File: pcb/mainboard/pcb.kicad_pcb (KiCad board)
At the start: 4 copper layers, 58 x 47 mm, 193 parts, among them J201 Conn_02x05_Odd_Even, J401 FH12-40S-0.5SH, J601 USB_C_Receptacle, SW701 EVQPUJ02K, U200 XC6SLX16-FTG256, U204 SY8008, U205 SY8008, U206 SY8008, U401 TPS65185, U502 MT41K64M16TW, U601 PTN3460, U602 TPS2001D, U603 USBLC6-2P6, U604 FUSB302BMPX, U605 CBTL02043A, U701 W25Q32JV, U702 RP2040, Y201 33MHz, Y701 12MHz

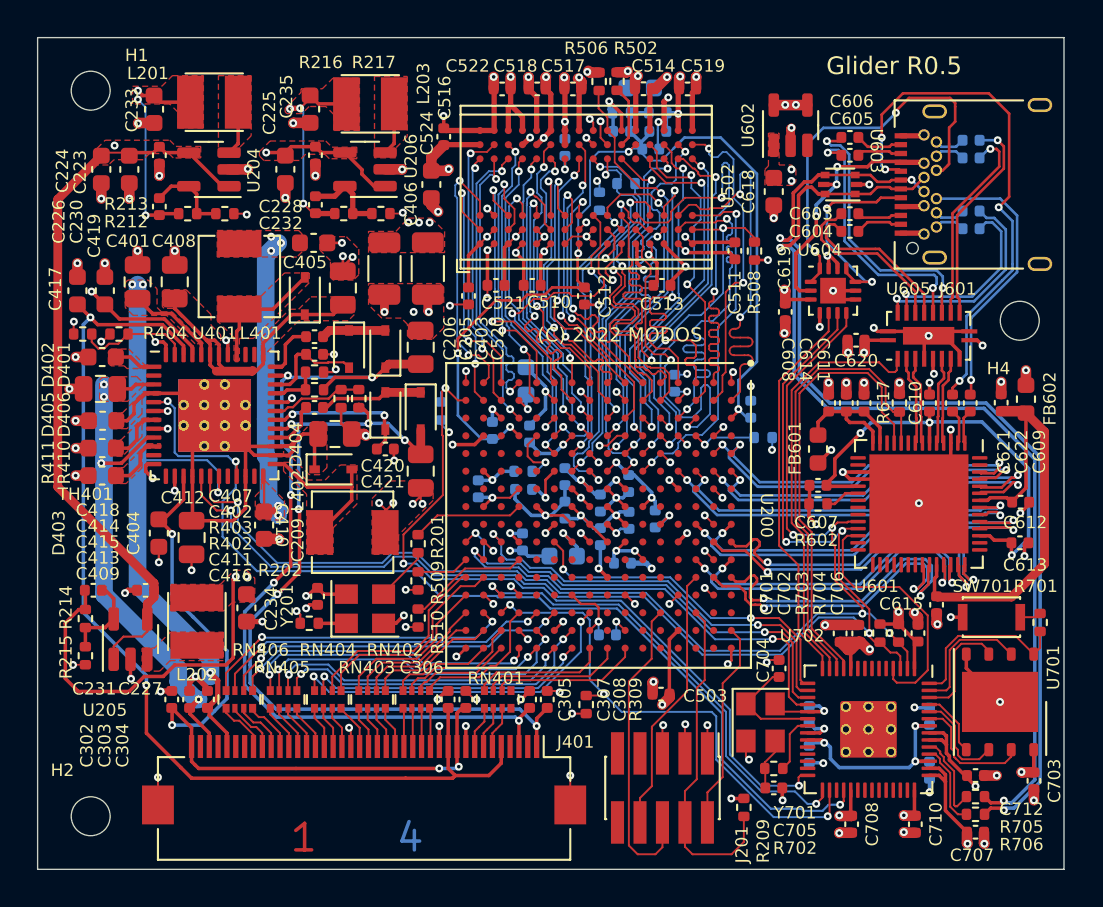
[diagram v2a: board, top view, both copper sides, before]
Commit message: pcb: r0p6
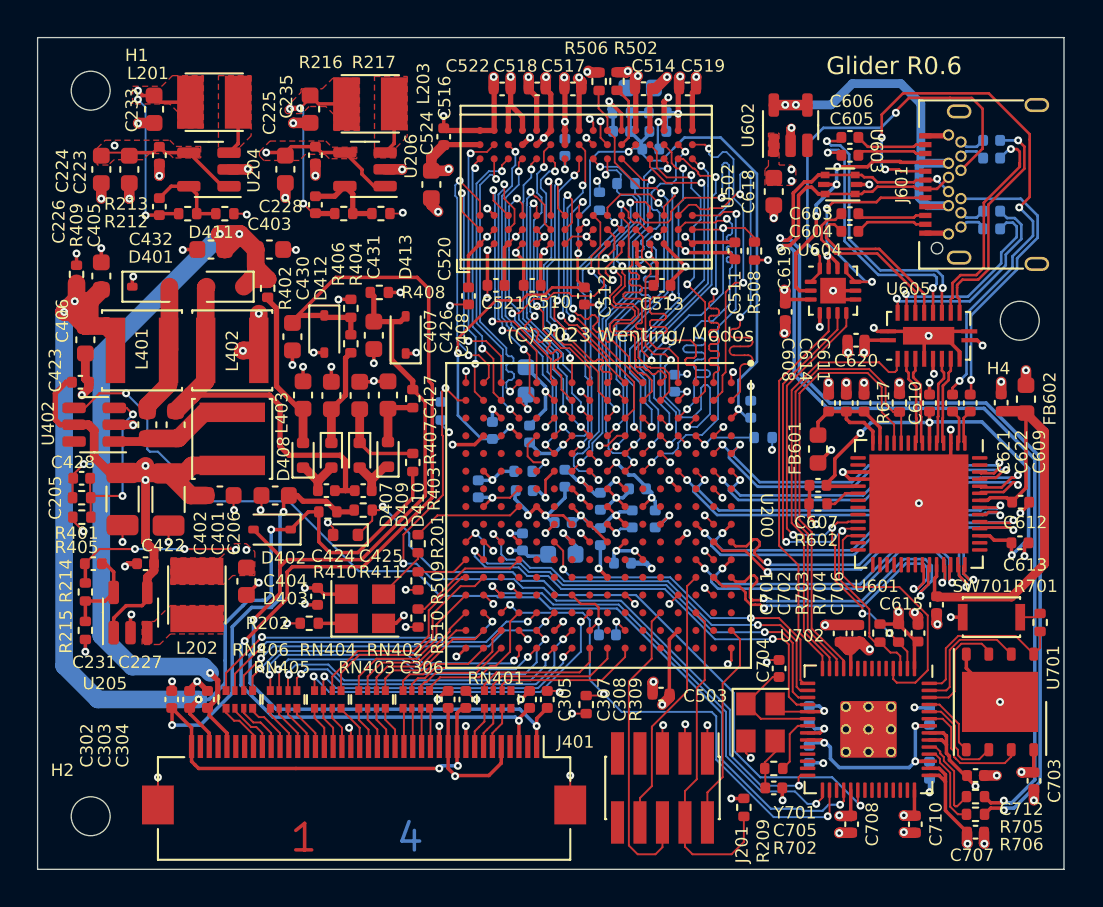
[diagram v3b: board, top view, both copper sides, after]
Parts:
- removed C409, C413, C414, C415, C417, C419: 4.7uF, Capacitor_SMD:C_0603_1608Metric
- removed C410: 10uF, Capacitor_SMD:C_0603_1608Metric
- removed C411: 10nF, Capacitor_SMD:C_0402_1005Metric
- removed C412, C416, C418, C421: 4.7uF/25V, Capacitor_SMD:C_0805_2012Metric
- removed C420: 100nF, Capacitor_SMD:C_0402_1005Metric
- removed D404, D405, D406: B0530WS, Diode_SMD:D_SOD-323
- removed TH401: 10K, Resistor_SMD:R_0402_1005Metric
- removed U401: TPS65185, footprints:QFN-48-1EP_7x7mm_P0.5mm_EP4.1x4.1mm_ThermalVias
- added C422: 10uF, Capacitor_SMD:C_0603_1608Metric, F.Cu at (110.3, 78.9)
- added C423: 100nF, Capacitor_SMD:C_0402_1005Metric, F.Cu at (102.4, 72.5)
- added C424: 10nF, Capacitor_SMD:C_0402_1005Metric, F.Cu at (116.3, 78.6)
- added C425: 10nF, Capacitor_SMD:C_0402_1005Metric, F.Cu at (118.4, 78.6)
- added C426: 1uF/50V, Capacitor_SMD:C_0603_1608Metric, F.Cu at (116.6, 73.2)
- added C427: 1uF/50V, Capacitor_SMD:C_0603_1608Metric, F.Cu at (119.8, 73.2)
- added C428: 22pF, Capacitor_SMD:C_0402_1005Metric, F.Cu at (102.5, 77.9)
- added C430: 1uF/50V, Capacitor_SMD:C_0603_1608Metric, F.Cu at (114.4, 69.9)
- added C431: 1uF/50V, Capacitor_SMD:C_0603_1608Metric, F.Cu at (119.0, 69.8)
- added C432: 10uF/25V, Capacitor_SMD:C_0603_1608Metric, F.Cu at (109.8, 65.0)
- added D407: 4148WT, Diode_SMD:D_SOD-523, F.Cu at (116.6, 76.6)
- added D408: 4148WT, Diode_SMD:D_SOD-523, F.Cu at (115.0, 76.6)
- added D409: 4148WT, Diode_SMD:D_SOD-523, F.Cu at (118.2, 76.6)
- added D410: 4148WT, Diode_SMD:D_SOD-523, F.Cu at (119.8, 76.5)
- added D411: B0530WS, Diode_SMD:D_SOD-323, F.Cu at (110.6, 67.1)
- added D412: EDZVT2R22B, Diode_SMD:D_SOD-323, F.Cu at (116.2, 69.8)
- added D413: EDZVT2R20B, Diode_SMD:D_SOD-323, F.Cu at (120.8, 69.8)
- added L403: WPN4020H2R2MT, Inductor_SMD:L_Changjiang_FNR4020S, F.Cu at (111.0, 75.7)
- added R401: 120K/1%, Resistor_SMD:R_0402_1005Metric, F.Cu at (102.5, 79.0)
- added R405: 5.1K/1%, Resistor_SMD:R_0402_1005Metric, F.Cu at (102.5, 80.1)
- added R406: 2K, Resistor_SMD:R_0402_1005Metric, F.Cu at (117.7, 70.3)
- added R407: 2K, Resistor_SMD:R_0402_1005Metric, F.Cu at (121.2, 73.4)
- added R408: 120K/1%, Resistor_SMD:R_0402_1005Metric, F.Cu at (119.3, 67.4)
- added R409: 120K/1%, Resistor_SMD:R_0402_1005Metric, F.Cu at (102.2, 66.4)
- added U402: SX1308, Package_TO_SOT_SMD:SOT-23-6, F.Cu at (103.2, 74.9)
- C401, C408: value 4.7uF/25V -> 1uF/50V; footprint Capacitor_SMD:C_0805_2012Metric -> Capacitor_SMD:C_0603_1608Metric
- C402: value 100nF -> 1uF/50V; footprint Capacitor_SMD:C_0402_1005Metric -> Capacitor_SMD:C_0603_1608Metric
- C403, C406: value 4.7uF/25V -> 10uF/25V; footprint Capacitor_SMD:C_0805_2012Metric -> Capacitor_SMD:C_0603_1608Metric
- C404: value 4.7uF -> 1uF/50V
- C405: value 10uF -> 10uF/25V
- C407: value 10nF -> 1uF/50V; footprint Capacitor_SMD:C_0402_1005Metric -> Capacitor_SMD:C_0603_1608Metric
- D403: value B0530WS -> 4148WT; footprint Diode_SMD:D_SOD-323 -> Diode_SMD:D_SOD-523
- J601: footprint Connector_USB:USB_C_Receptacle_Amphenol_12401548E4-2A -> footprints:USB-306A-B-SU
- L401: value FXL0420-2R2-M -> WPN4020H100MT; footprint footprints:L_FXL0420 -> Inductor_SMD:L_Changjiang_FNR4020S
- L402: value FXL0420-4R7-M -> WPN4020H100MT; footprint footprints:L_FXL0420 -> Inductor_SMD:L_Changjiang_FNR4020S
- R212: value 121K/1% -> 120K/1%
- R214: value 22.6K/1% -> 20K/1%
- R215: value 27K/1% -> 24K/1%
- R216: value 34.8K/1% -> 24K/1%
- R217: value 27K/1% -> 20K/1%
- R402: value 470K/1% -> 2K
- R403: value 18K/1% -> 0
- R404: value 43K -> 120K/1%
- R410: value 510K/1% -> 18K/1%
- R411: value 24K/1% -> 5.1K/1%
- moved C205 21.6 mm to (104.8, 79.1)
- moved C206 17.9 mm to (107.4, 79.1)
- moved C406 14.8 mm to (102.7, 70.1)
- moved D401 13.7 mm to (106.4, 67.1), turned to 0 degrees
- moved D403 13.7 mm to (117.4, 81.1), turned to 180 degrees
- moved R404 13.2 mm to (117.7, 68.3), turned to -90 degrees
- moved L402 12.3 mm to (111.0, 70.7), turned to 180 degrees
- moved C408 12.3 mm to (118.2, 73.2), turned to 90 degrees
- moved C405 12.1 mm to (103.6, 66.5), turned to 90 degrees
- moved D402 11.1 mm to (113.2, 80.8), turned to 180 degrees
- moved C402 10.3 mm to (106.2, 74.9), turned to 90 degrees
- moved C403 10.2 mm to (113.1, 65.0), turned to 0 degrees
- moved C401 8.36 mm to (107.8, 74.9), turned to 90 degrees
- moved R403 7.54 mm to (121.2, 77.0), turned to 90 degrees
- moved C404 6.91 mm to (113.4, 78.9), turned to 0 degrees
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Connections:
- C306 pad 1: +3V3_LCD -> +3V3
- C401 pad 1: GND -> Net-(U402-SW)
- C401 pad 2: VPOS -> Net-(D411-A)
- C402 pad 1: GND -> Net-(U402-SW)
- C402 pad 2: Net-(D402-Pad2) -> Net-(D401-A)
- C403 pad 1: GND -> VPOS
- C403 pad 2: VGH -> GND
- C405 pad 1: GND -> VNEG
- C405 pad 2: +5V -> GND
- C406 pad 1: GND -> VNEG
- C406 pad 2: Net-(C406-Pad2) -> GND
- C407 pad 1: Net-(C407-Pad1) -> GND
- C407 pad 2: Net-(C407-Pad2) -> Net-(D408-A)
- C408 pad 1: GND -> Net-(D409-K)
- C408 pad 2: Net-(C406-Pad2) -> GND
- D401 pad 1: VGH -> GND
- D401 pad 2: Net-(C407-Pad1) -> Net-(D401-A)
- D402 pad 1: Net-(C407-Pad1) -> VNEG
- D402 pad 2: Net-(D402-Pad2) -> VGL
- D403 pad 1: Net-(C406-Pad2) -> EPD_VCOM_PWM
- D403 pad 2: Net-(L401-Pad2) -> GND
- J401 pad 11: +3V3_LCD -> +3V3
- J401 pad 5: +3V3_LCD -> +3V3
- L401 pad 1: +5V -> Net-(D401-A)
- L401 pad 2: Net-(L401-Pad2) -> VNEG
- L402 pad 1: Net-(D404-Pad2) -> GND
- L402 pad 2: GND -> Net-(D411-A)
- R402 pad 1: VGH -> VPOS
- R402 pad 2: Net-(R402-Pad2) -> Net-(D408-A)
- R403 pad 1: Net-(R402-Pad2) -> VNEG
- R403 pad 2: GND -> Net-(D409-K)
- R404 pad 2: Net-(R404-Pad2) -> VGH
- R410 pad 1: VGL -> VNEG
- R410 pad 2: Net-(R410-Pad2) -> VCOM
- R411 pad 1: Net-(R410-Pad2) -> VCOM
- R411 pad 2: GND -> EPD_VCOM_PWM
- U702 pad 34: /mcu/GPIO22 -> EPD_VCOM_PWM
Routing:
- net +3V3_LCD: track 59.0 -> 0.00 mm, vias 2 -> 0
- net I2C_SCL: track 73.1 -> 28.3 mm, vias 4 -> 2
- net I2C_SDA: track 71.7 -> 28.0 mm, vias 5 -> 4
- net EPD_VCOM_PWM: track 0.00 -> 39.7 mm, vias 0 -> 2
- net VNEG: track 29.2 -> 67.4 mm
- net Net-(C415-Pad1): track 34.4 -> 0.00 mm
- net +5V: track 69.3 -> 45.0 mm, vias 12 -> 6
- net Net-(D411-A): track 0.00 -> 22.1 mm
- net Net-(C406-Pad2): track 19.1 -> 0.00 mm
- net /dp_in/VBUS: track 19.6 -> 37.8 mm
- net VGH: track 49.4 -> 61.9 mm, vias 5 -> 2
- net +1V1: track 37.3 -> 26.3 mm, vias 7 -> 9
- net Net-(U402-FB): track 0.00 -> 10.1 mm, vias 0 -> 2
- net Net-(D408-A): track 0.00 -> 9.19 mm
- net Net-(D404-Pad2): track 9.15 -> 0.00 mm
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- removed copper zone on F.Cu, net GND
- removed copper zone on F.Cu, net IPSOUT
- removed copper zone on F.Cu, net Net-(C406-Pad2)
- removed copper zone on F.Cu, net Net-(C413-Pad1)
- removed copper zone on F.Cu, net Net-(C414-Pad1)
- removed copper zone on F.Cu, net Net-(C415-Pad1)
- removed copper zone on F.Cu, net Net-(D404-Pad2)
- removed copper zone on F.Cu, net Net-(L401-Pad2)
- removed copper zone on F.Cu, net VNEG
- removed copper zone on F.Cu, net VPOS
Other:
- board text added: "(C) 2023 Wenting/ Modos"
- board text added: "Glider R0.6"
- board text removed: "(C) 2022 MODOS"
- board text removed: "Glider R0.5"

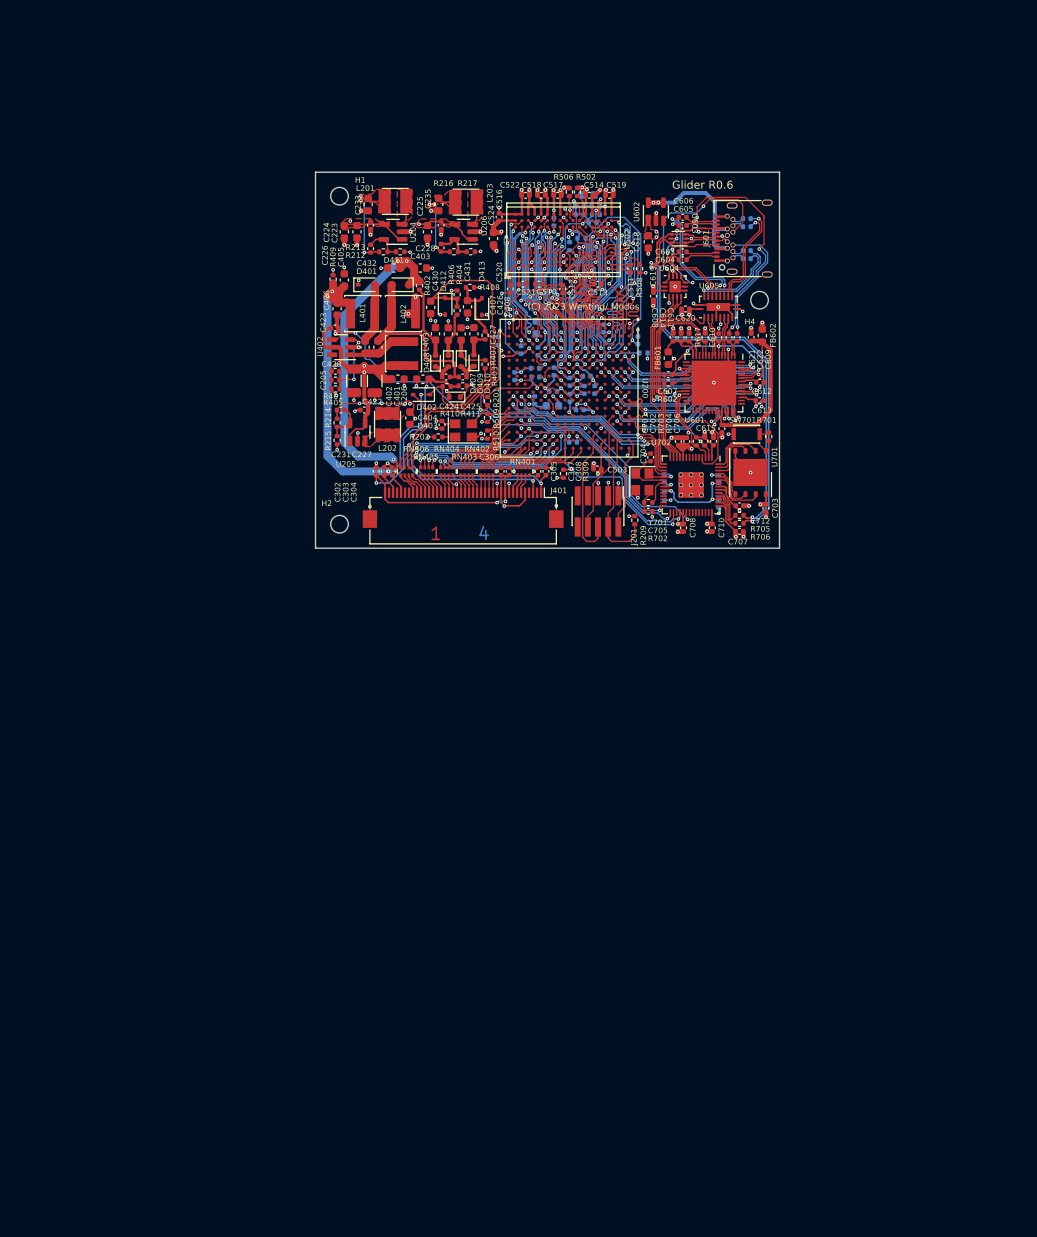
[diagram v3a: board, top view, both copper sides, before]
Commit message: r0p7 wip, check in before switch to kicad 8
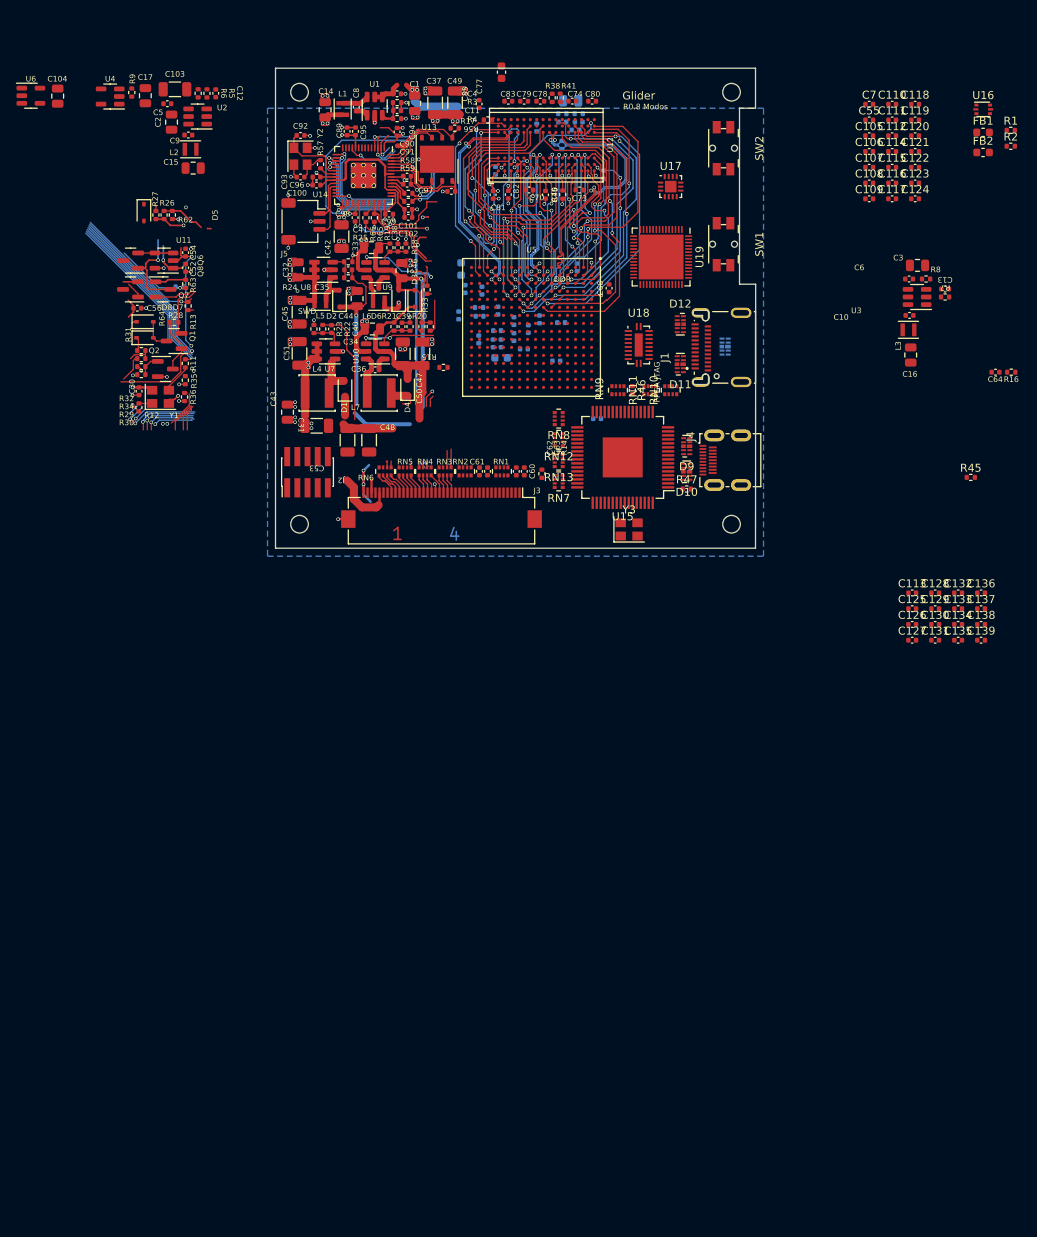
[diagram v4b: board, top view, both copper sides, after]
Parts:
- removed C205, C206: 100uF/6.3V, Capacitor_SMD:C_1206_3216Metric
- removed C223, C224, C225, C233, C234, C235, C422, C618: 10uF, Capacitor_SMD:C_0603_1608Metric
- removed C226, C227, C228, C423, C601, C602, C603, C604, C605, C606, C610, C611, C612, C613, C614, C615, C616, C617, C619, C620, C621, C622, C702, C703, C706, C707, C708, C709, C710, C711, C712, C713: 100nF, Capacitor_SMD:C_0402_1005Metric
- removed C230, C231, C232, C302, C303, C304: 220nF, Capacitor_SMD:C_0402_1005Metric
- removed C401, C402, C404, C407, C408, C426, C427, C430, C431: 1uF/50V, Capacitor_SMD:C_0603_1608Metric
- removed C403, C405, C406, C432: 10uF/25V, Capacitor_SMD:C_0603_1608Metric
- removed C424, C425: 10nF, Capacitor_SMD:C_0402_1005Metric
- removed C428: 22pF, Capacitor_SMD:C_0402_1005Metric
- removed C607, C608, C609, C701, C714: 1uF, Capacitor_SMD:C_0402_1005Metric
- removed C704, C705: 18pF, Capacitor_SMD:C_0402_1005Metric
- removed D401, D402, D411: B0530WS, Diode_SMD:D_SOD-323
- removed D403, D407, D408, D409, D410: 4148WT, Diode_SMD:D_SOD-523
- removed D412: EDZVT2R22B, Diode_SMD:D_SOD-323
- removed D413: EDZVT2R20B, Diode_SMD:D_SOD-323
- removed FB601, FB602: 120, Inductor_SMD:L_0603_1608Metric
- removed J601: USB_C_Receptacle, footprints:USB-306A-B-SU
- removed L201, L202, L203: 4.7uH, footprints:L_1212
- removed L401, L402: WPN4020H100MT, Inductor_SMD:L_Changjiang_FNR4020S
- removed L403: WPN4020H2R2MT, Inductor_SMD:L_Changjiang_FNR4020S
- removed R212, R401, R404, R408, R409: 120K/1%, Resistor_SMD:R_0402_1005Metric
- removed R213: 27K/1%, Resistor_SMD:R_0402_1005Metric
- removed R214, R217: 20K/1%, Resistor_SMD:R_0402_1005Metric
- removed R215, R216: 24K/1%, Resistor_SMD:R_0402_1005Metric
- removed R402, R406, R407: 2K, Resistor_SMD:R_0402_1005Metric
- removed R403: 0, Resistor_SMD:R_0402_1005Metric
- removed R405, R411: 5.1K/1%, Resistor_SMD:R_0402_1005Metric
- removed R410: 18K/1%, Resistor_SMD:R_0402_1005Metric
- removed R602, R617, R703, R704: 4.7K, Resistor_SMD:R_0402_1005Metric
- removed R701, R702: 1K, Resistor_SMD:R_0402_1005Metric
- removed R705, R706: 27, Resistor_SMD:R_0402_1005Metric
- removed SW701: EVQPUJ02K, Button_Switch_SMD:SW_SPST_CK_KXT3
- removed U204, U205, U206: SY8008, Package_TO_SOT_SMD:TSOT-23-5
- removed U402: SX1308, Package_TO_SOT_SMD:SOT-23-6
- removed U601: PTN3460, Package_DFN_QFN:QFN-56-1EP_7x7mm_P0.4mm_EP5.6x5.6mm
- removed U602: TPS2001D, Package_TO_SOT_SMD:SOT-23-5
- removed U603: USBLC6-2P6, Package_TO_SOT_SMD:SOT-666
- removed U604: FUSB302BMPX, Package_DFN_QFN:WQFN-14-1EP_2.5x2.5mm_P0.5mm_EP1.45x1.45mm
- removed U605: CBTL02043A, Package_DFN_QFN:WQFN-20-1EP_2.5x4.5mm_P0.5mm_EP1x2.9mm
- removed U701: W25Q32JV, Package_SON:WSON-8-1EP_6x5mm_P1.27mm_EP3.4x4.3mm
- removed U702: RP2040, footprints:RP2040-QFN-56
- removed Y701: 12MHz, Oscillator:Oscillator_SMD_Abracon_ASE-4Pin_3.2x2.5mm
- added C1: 10uF/10V, Capacitor_SMD:C_0805_2012Metric, F.Cu at (112.4, 44.4)
- added C10: 100nF, Capacitor_SMD:C_0402_1005Metric, F.Cu at (174.2, 70.9)
- added C100: 100nF, Capacitor_SMD:C_0402_1005Metric, F.Cu at (100.1, 54.6)
- added C101: 100nF, Capacitor_SMD:C_0402_1005Metric, F.Cu at (111.6, 57.6)
- added C102: 1uF, Capacitor_SMD:C_0402_1005Metric, F.Cu at (111.6, 58.6)
- added C103: 47uF/10V, Capacitor_SMD:C_1206_3216Metric, F.Cu at (82.4, 42.6)
- added C104: 10uF/10V, Capacitor_SMD:C_0805_2012Metric, F.Cu at (67.8, 43.5)
- added C105: 100nF, Capacitor_SMD:C_0402_1005Metric, F.Cu at (169.2, 48.4)
- added C106: 100nF, Capacitor_SMD:C_0402_1005Metric, F.Cu at (169.2, 50.4)
- added C107: 100nF, Capacitor_SMD:C_0402_1005Metric, F.Cu at (169.2, 52.4)
- added C108: 100nF, Capacitor_SMD:C_0402_1005Metric, F.Cu at (169.2, 54.4)
- added C109: 100nF, Capacitor_SMD:C_0402_1005Metric, F.Cu at (169.2, 56.3)
- added C11: 47pF, Capacitor_SMD:C_0402_1005Metric, F.Cu at (110.2, 45.3)
- added C110: 100nF, Capacitor_SMD:C_0402_1005Metric, F.Cu at (172.1, 44.5)
- added C111: 100nF, Capacitor_SMD:C_0402_1005Metric, F.Cu at (172.1, 46.5)
- added C112: 100nF, Capacitor_SMD:C_0402_1005Metric, F.Cu at (172.1, 48.4)
- added C113: 18pF, Capacitor_SMD:C_0402_1005Metric, F.Cu at (174.6, 105.6)
- added C114: 100nF, Capacitor_SMD:C_0402_1005Metric, F.Cu at (172.1, 50.4)
- added C115: 100nF, Capacitor_SMD:C_0402_1005Metric, F.Cu at (172.1, 52.4)
- added C116: 1uF, Capacitor_SMD:C_0402_1005Metric, F.Cu at (172.1, 54.4)
- added C117: 1uF, Capacitor_SMD:C_0402_1005Metric, F.Cu at (172.1, 56.3)
- added C118: 1uF, Capacitor_SMD:C_0402_1005Metric, F.Cu at (175.0, 44.5)
- added C119: 100nF, Capacitor_SMD:C_0402_1005Metric, F.Cu at (175.0, 46.5)
- added C12: 47pF, Capacitor_SMD:C_0402_1005Metric, F.Cu at (87.5, 43.1)
- added C120: 100nF, Capacitor_SMD:C_0402_1005Metric, F.Cu at (175.0, 48.4)
- added C121: 100nF, Capacitor_SMD:C_0402_1005Metric, F.Cu at (175.0, 50.4)
- added C122: 100nF, Capacitor_SMD:C_0402_1005Metric, F.Cu at (175.0, 52.4)
- added C123: 100nF, Capacitor_SMD:C_0402_1005Metric, F.Cu at (175.0, 54.4)
- added C124: 100nF, Capacitor_SMD:C_0402_1005Metric, F.Cu at (175.0, 56.3)
- added C125: 18pF, Capacitor_SMD:C_0402_1005Metric, F.Cu at (174.6, 107.6)
- added C126: 1uF, Capacitor_SMD:C_0402_1005Metric, F.Cu at (174.6, 109.5)
- added C127: 100nF, Capacitor_SMD:C_0402_1005Metric, F.Cu at (174.6, 111.5)
- added C128: 100nF, Capacitor_SMD:C_0402_1005Metric, F.Cu at (177.5, 105.6)
- added C129: 100nF, Capacitor_SMD:C_0402_1005Metric, F.Cu at (177.5, 107.6)
- added C13: 47pF, Capacitor_SMD:C_0402_1005Metric, F.Cu at (178.7, 67.6)
- added C130: 100nF, Capacitor_SMD:C_0402_1005Metric, F.Cu at (177.5, 109.5)
- added C131: 100nF, Capacitor_SMD:C_0402_1005Metric, F.Cu at (177.5, 111.5)
- added C132: 1uF, Capacitor_SMD:C_0402_1005Metric, F.Cu at (180.3, 105.6)
- added C133: 100nF, Capacitor_SMD:C_0402_1005Metric, F.Cu at (180.3, 107.6)
- added C134: 100nF, Capacitor_SMD:C_0402_1005Metric, F.Cu at (180.3, 109.5)
- added C135: 100nF, Capacitor_SMD:C_0402_1005Metric, F.Cu at (180.3, 111.5)
- added C136: 100nF, Capacitor_SMD:C_0402_1005Metric, F.Cu at (183.2, 105.6)
- added C137: 100nF, Capacitor_SMD:C_0402_1005Metric, F.Cu at (183.2, 107.6)
- added C138: 100nF, Capacitor_SMD:C_0402_1005Metric, F.Cu at (183.2, 109.5)
- added C139: 100nF, Capacitor_SMD:C_0402_1005Metric, F.Cu at (183.2, 111.5)
- added C14: 10uF/10V, Capacitor_SMD:C_0805_2012Metric, F.Cu at (101.2, 45.2)
- added C15: 10uF/10V, Capacitor_SMD:C_0805_2012Metric, F.Cu at (84.7, 52.5)
- added C16: 10uF/10V, Capacitor_SMD:C_0805_2012Metric, F.Cu at (174.4, 75.8)
- added C17: 10uF/10V, Capacitor_SMD:C_0805_2012Metric, F.Cu at (78.7, 43.4)
- added C2: 10uF/10V, Capacitor_SMD:C_0805_2012Metric, F.Cu at (82.0, 46.7)
- added C3: 10uF/10V, Capacitor_SMD:C_0805_2012Metric, F.Cu at (175.2, 64.7)
- added C31: 10uF/10V, Capacitor_SMD:C_0805_2012Metric, F.Cu at (96.5, 83.0)
- added C32: 10uF/10V, Capacitor_SMD:C_0805_2012Metric, F.Cu at (97.8, 65.2)
- added C33: 4.7uF/50V, Capacitor_SMD:C_0805_2012Metric, F.Cu at (107.0, 62.4)
- added C34: 4.7uF/50V, Capacitor_SMD:C_0805_2012Metric, F.Cu at (107.1, 72.6)
- added C35: 100nF, Capacitor_SMD:C_0402_1005Metric, F.Cu at (107.4, 67.5)
- added C36: 100nF, Capacitor_SMD:C_0402_1005Metric, F.Cu at (107.5, 77.7)
- added C37: 47uF/10V, Capacitor_SMD:C_1206_3216Metric, F.Cu at (115.0, 44.3)
- added C38: 22pF, Capacitor_SMD:C_0402_1005Metric, F.Cu at (110.3, 62.4)
- added C39: 22pF, Capacitor_SMD:C_0402_1005Metric, F.Cu at (110.8, 72.3)
- added C4: 100nF, Capacitor_SMD:C_0402_1005Metric, F.Cu at (110.2, 43.2)
- added C40: 22pF, Capacitor_SMD:C_0402_1005Metric, F.Cu at (102.0, 72.6)
- added C41: 22pF, Capacitor_SMD:C_0402_1005Metric, F.Cu at (104.1, 65.2)
- added C42: 47uF/10V, Capacitor_SMD:C_1206_3216Metric, F.Cu at (103.2, 61.0)
- added C43: 10uF/50V, Capacitor_SMD:C_1206_3216Metric, F.Cu at (104.0, 86.5)
- added C44: 4.7uF/50V, Capacitor_SMD:C_0805_2012Metric, F.Cu at (105.2, 68.8)
- added C45: 47uF/10V, Capacitor_SMD:C_1206_3216Metric, F.Cu at (98.0, 70.5)
- added C46: 4.7uF/50V, Capacitor_SMD:C_0805_2012Metric, F.Cu at (110.8, 65.3)
- added C47: 10uF/50V, Capacitor_SMD:C_1206_3216Metric, F.Cu at (110.9, 75.7)
- added C48: 10uF/50V, Capacitor_SMD:C_1206_3216Metric, F.Cu at (106.7, 86.5)
- added C49: 47uF/10V, Capacitor_SMD:C_1206_3216Metric, F.Cu at (117.4, 44.3)
- added C5: 100nF, Capacitor_SMD:C_0402_1005Metric, F.Cu at (81.5, 44.4)
- added C50: 10uF/50V, Capacitor_SMD:C_1206_3216Metric, F.Cu at (113.4, 75.7)
- added C51: 47uF/10V, Capacitor_SMD:C_1206_3216Metric, F.Cu at (98.0, 75.7)
- added C52: 220nF, Capacitor_SMD:C_0402_1005Metric, F.Cu at (83.8, 65.0)
- added C53: 47uF/10V, Capacitor_SMD:C_1206_3216Metric, F.Cu at (100.2, 84.7)
- added C54: 100nF, Capacitor_SMD:C_0402_1005Metric, F.Cu at (83.8, 63.0)
- added C55: 100nF, Capacitor_SMD:C_0402_1005Metric, F.Cu at (169.2, 46.5)
- added C56: 1uF, Capacitor_SMD:C_0402_1005Metric, F.Cu at (77.7, 70.0)
- added C57: 220nF, Capacitor_SMD:C_0402_1005Metric, B.Cu at (130.1, 76.6)
- added C58: 220nF, Capacitor_SMD:C_0402_1005Metric, B.Cu at (123.2, 74.4)
- added C59: 220nF, Capacitor_SMD:C_0402_1005Metric, B.Cu at (122.2, 74.4)
- added C6: 100nF, Capacitor_SMD:C_0402_1005Metric, F.Cu at (174.2, 66.3)
- added C7: 100nF, Capacitor_SMD:C_0402_1005Metric, F.Cu at (169.2, 44.5)
- added C8: 100nF, Capacitor_SMD:C_0402_1005Metric, F.Cu at (105.1, 44.9)
- added C89: 1uF, Capacitor_SMD:C_0402_1005Metric, F.Cu at (104.0, 47.9)
- added C9: 100nF, Capacitor_SMD:C_0402_1005Metric, F.Cu at (84.1, 48.4)
- added C90: 100nF, Capacitor_SMD:C_0402_1005Metric, F.Cu at (111.5, 53.5)
- added C91: 100nF, Capacitor_SMD:C_0402_1005Metric, F.Cu at (111.5, 54.5)
- added C92: 18pF, Capacitor_SMD:C_0402_1005Metric, F.Cu at (98.1, 48.4)
- added C93: 18pF, Capacitor_SMD:C_0402_1005Metric, F.Cu at (98.1, 53.6)
- added C94: 100nF, Capacitor_SMD:C_0402_1005Metric, F.Cu at (110.2, 48.0)
- added C95: 100nF, Capacitor_SMD:C_0402_1005Metric, F.Cu at (105.0, 47.9)
- added C96: 100nF, Capacitor_SMD:C_0402_1005Metric, F.Cu at (100.1, 53.6)
- added C97: 100nF, Capacitor_SMD:C_0402_1005Metric, F.Cu at (117.0, 55.4)
- added C98: 100nF, Capacitor_SMD:C_0402_1005Metric, F.Cu at (105.0, 58.7)
- added C99: 100nF, Capacitor_SMD:C_0402_1005Metric, F.Cu at (109.2, 58.2)
- added D1: 1N5819WS, Diode_SMD:D_SOD-323, F.Cu at (103.7, 80.0)
- added D10: RCLAMP0524P, Package_DFN_QFN:Diodes_UDFN-10_1.0x2.5mm_P0.5mm, F.Cu at (146.4, 90.5)
- added D11: RCLAMP0524P, Package_DFN_QFN:Diodes_UDFN-10_1.0x2.5mm_P0.5mm, F.Cu at (145.6, 77.0)
- added D12: RCLAMP0524P, Package_DFN_QFN:Diodes_UDFN-10_1.0x2.5mm_P0.5mm, F.Cu at (145.6, 72.0)
- added D13: RCLAMP0524P, Package_DFN_QFN:Diodes_UDFN-10_1.0x2.5mm_P0.5mm, B.Cu at (151.2, 74.8)
- added D2: 1N5819WS, Diode_SMD:D_SOD-323, F.Cu at (103.0, 68.8)
- added D3: 1N5819WS, Diode_SMD:D_SOD-323, F.Cu at (110.4, 68.8)
- added D4: 1N5819WS, Diode_SMD:D_SOD-323, F.Cu at (111.5, 79.9)
- added D5: 4148WS, Diode_SMD:D_SOD-323, F.Cu at (78.5, 58.0)
- added D6: 1N5819WS, Diode_SMD:D_SOD-323, F.Cu at (112.4, 68.8)
- added D7: 4148WS, Diode_SMD:D_SOD-323, F.Cu at (78.7, 71.7)
- added D8: 4148WS, Diode_SMD:D_SOD-323, F.Cu at (78.7, 73.7)
- added D9: RCLAMP0524P, Package_DFN_QFN:Diodes_UDFN-10_1.0x2.5mm_P0.5mm, F.Cu at (146.4, 87.2)
- added FB1: 120, Inductor_SMD:L_0603_1608Metric, F.Cu at (183.4, 48.0)
- added FB2: 120, Inductor_SMD:L_0603_1608Metric, F.Cu at (183.4, 50.5)
- added H3: MountingHole, MountingHole:MountingHole_2.2mm_M2_DIN965, F.Cu at (152.0, 97.0)
- added J1: USB_C_Receptacle, footprints:AMPHENOL_10137065-00021LF, F.Cu at (153.2, 74.9)
- added J4: DVI, Connector_HDMI:HDMI_Micro-D_Molex_46765-1x01, F.Cu at (153.2, 89.0)
- added J5: SM03B-SRSS-TB, Connector_JST:JST_SH_SM03B-SRSS-TB_1x03-1MP_P1.00mm_Horizontal, F.Cu at (98.5, 59.1)
- added L1: FTC201610S4R7MBCA, Inductor_SMD:L_Murata_DFE201610P, F.Cu at (103.4, 45.1)
- added L2: FTC201610S4R7MBCA, Inductor_SMD:L_Murata_DFE201610P, F.Cu at (84.4, 50.1)
- added L3: FTC201610S4R7MBCA, Inductor_SMD:L_Murata_DFE201610P, F.Cu at (174.1, 72.7)
- added L4: WPN4020H4R7MT, Inductor_SMD:L_Changjiang_FNR4020S, F.Cu at (100.2, 80.6)
- added L5: FTC201610S4R7MBCA, Inductor_SMD:L_Murata_DFE201610P, F.Cu at (100.6, 69.2)
- added L6: FTC201610S4R7MBCA, Inductor_SMD:L_Murata_DFE201610P, F.Cu at (107.9, 69.2)
- added L7: WPN4020H4R7MT, Inductor_SMD:L_Changjiang_FNR4020S, F.Cu at (108.0, 80.6)
- added Q1: AO3401A, Package_TO_SOT_SMD:SOT-23, F.Cu at (82.3, 74.1)
- added Q2: S8050, Package_TO_SOT_SMD:SOT-23, F.Cu at (81.2, 77.6)
- added Q6: AO3400A, Package_TO_SOT_SMD:SOT-23, F.Cu at (76.9, 64.0)
- added Q7: AO3401A, Package_TO_SOT_SMD:SOT-23, F.Cu at (80.9, 67.7)
- added Q8: AO3401A, Package_TO_SOT_SMD:SOT-23, F.Cu at (76.9, 67.7)
- added R1: 4.7K, Resistor_SMD:R_0402_1005Metric, F.Cu at (186.9, 47.8)
- added R15: 1K/1%, Resistor_SMD:R_0402_1005Metric, F.Cu at (116.0, 77.4)
- added R17: 10K/1%, Resistor_SMD:R_0402_1005Metric, F.Cu at (121.5, 46.5)
- added R18: 240K/1%, Resistor_SMD:R_0402_1005Metric, F.Cu at (111.3, 62.4)
- added R19: 10K/1%, Resistor_SMD:R_0402_1005Metric, F.Cu at (109.3, 62.4)
- added R2: 4.7K, Resistor_SMD:R_0402_1005Metric, F.Cu at (186.9, 49.8)
- added R20: 91K/1%, Resistor_SMD:R_0402_1005Metric, F.Cu at (111.8, 72.3)
- added R21: 5.1K/1%, Resistor_SMD:R_0402_1005Metric, F.Cu at (109.8, 72.3)
- added R22: 240K/1%, Resistor_SMD:R_0402_1005Metric, F.Cu at (100.9, 72.6)
- added R23: 10K/1%, Resistor_SMD:R_0402_1005Metric, F.Cu at (99.8, 72.6)
- added R24: 360K/1%, Resistor_SMD:R_0402_1005Metric, F.Cu at (104.1, 66.2)
- added R25: 10K/1%, Resistor_SMD:R_0402_1005Metric, F.Cu at (104.1, 64.2)
- added R26: 91K/1%, Resistor_SMD:R_0402_1005Metric, F.Cu at (81.1, 58.4)
- added R27: 27K/1%, Resistor_SMD:R_0402_1005Metric, F.Cu at (80.0, 58.4)
- added R28: 120K/1%, Resistor_SMD:R_0402_1005Metric, F.Cu at (82.3, 71.8)
- added R29: 5.1K/1%, Resistor_SMD:R_0402_1005Metric, F.Cu at (78.2, 77.3)
- added R3: 91K/1%, Resistor_SMD:R_0402_1005Metric, F.Cu at (110.2, 44.3)
- added R30: 27K/1%, Resistor_SMD:R_0402_1005Metric, F.Cu at (78.2, 78.3)
- added R31: 120K/1%, Resistor_SMD:R_0402_1005Metric, F.Cu at (114.3, 72.3)
- added R32: 120K/1%, Resistor_SMD:R_0402_1005Metric, F.Cu at (78.2, 75.3)
- added R33: 120K/1%, Resistor_SMD:R_0402_1005Metric, F.Cu at (113.3, 72.3)
- added R34: 120K/1%, Resistor_SMD:R_0402_1005Metric, F.Cu at (78.2, 76.3)
- added R4: 20K/1%, Resistor_SMD:R_0402_1005Metric, F.Cu at (110.2, 46.3)
- added R45: 1M, Resistor_SMD:R_0402_1005Metric, F.Cu at (181.9, 91.2)
- added R46: 33, Resistor_SMD:R_0402_1005Metric, F.Cu at (139.6, 80.2)
- added R47: 10K, Resistor_SMD:R_0402_1005Metric, F.Cu at (146.4, 92.6)
- added R5: 20K/1%, Resistor_SMD:R_0402_1005Metric, F.Cu at (86.4, 43.1)
- added R56: 1K, Resistor_SMD:R_0402_1005Metric, F.Cu at (117.4, 47.5)
- added R57: 1K, Resistor_SMD:R_0402_1005Metric, F.Cu at (100.6, 52.0)
- added R58: 27R, Resistor_SMD:R_0402_1005Metric, F.Cu at (111.6, 55.6)
- added R59: 27R, Resistor_SMD:R_0402_1005Metric, F.Cu at (111.6, 56.6)
- added R6: 16K/1%, Resistor_SMD:R_0402_1005Metric, F.Cu at (85.3, 43.1)
- added R62: 120K/1%, Resistor_SMD:R_0402_1005Metric, F.Cu at (82.1, 58.4)
- added R63: 51R, Resistor_SMD:R_0402_1005Metric, F.Cu at (83.8, 67.0)
- added R64: 20K/1%, Resistor_SMD:R_0402_1005Metric, F.Cu at (114.0, 67.7)
- added R65: 10K/1%, Resistor_SMD:R_0402_1005Metric, F.Cu at (107.3, 58.7)
- added R66: 51R, Resistor_SMD:R_0402_1005Metric, F.Cu at (106.3, 58.7)
- added R7: 16K/1%, Resistor_SMD:R_0402_1005Metric, F.Cu at (178.7, 68.6)
- added R8: 27K/1%, Resistor_SMD:R_0402_1005Metric, F.Cu at (176.3, 66.3)
- added R9: 10K/1%, Resistor_SMD:R_0402_1005Metric, F.Cu at (77.0, 43.0)
- added RN10: 33R / 4D02WGF330JTCE, Resistor_SMD:R_Array_Convex_4x0402, F.Cu at (144.4, 80.2)
- added RN11: 33R / 4D02WGF330JTCE, Resistor_SMD:R_Array_Convex_4x0402, F.Cu at (141.8, 80.2)
- added RN12: 33R / 4D02WGF330JTCE, Resistor_SMD:R_Array_Convex_4x0402, F.Cu at (130.4, 86.5)
- added RN13: 33R / 4D02WGF330JTCE, Resistor_SMD:R_Array_Convex_4x0402, F.Cu at (130.4, 89.0)
- added RN7: 33R / 4D02WGF330JTCE, Resistor_SMD:R_Array_Convex_4x0402, F.Cu at (130.4, 91.7)
- added RN8: 33R / 4D02WGF330JTCE, Resistor_SMD:R_Array_Convex_4x0402, F.Cu at (130.4, 83.8)
- added RN9: 33R / 4D02WGF330JTCE, Resistor_SMD:R_Array_Convex_4x0402, F.Cu at (137.8, 80.2)
- added SW1: SW, Button_Switch_SMD:Panasonic_EVQPUL_EVQPUC, F.Cu at (151.0, 62.0)
- added SW2: SW, Button_Switch_SMD:Panasonic_EVQPUL_EVQPUC, F.Cu at (151.0, 50.0)
- added U1: SY8120, Package_TO_SOT_SMD:TSOT-23-6, F.Cu at (107.4, 44.7)
- added U10: LGS5148, Package_TO_SOT_SMD:TSOT-23-6, F.Cu at (107.5, 75.4)
- added U11: LM321, Package_TO_SOT_SMD:SOT-23-5, F.Cu at (81.1, 64.0)
- added U13: W25Q32JV, Package_SON:WSON-8-1EP_6x5mm_P1.27mm_EP3.4x4.3mm, F.Cu at (115.2, 51.4)
- added U14: RP2040, footprints:RP2040-QFN-56, F.Cu at (106.0, 53.4)
- added U15: ADV7611, Package_QFP:LQFP-64-1EP_10x10mm_P0.5mm_EP5x5mm, F.Cu at (138.4, 88.7)
- added U16: USBLC6-2P6, Package_TO_SOT_SMD:SOT-666, F.Cu at (183.5, 45.1)
- added U17: FUSB302BMPX, Package_DFN_QFN:WQFN-14-1EP_2.5x2.5mm_P0.5mm_EP1.45x1.45mm, F.Cu at (144.4, 54.8)
- added U18: CBTL02043A, Package_DFN_QFN:WQFN-20-1EP_2.5x4.5mm_P0.5mm_EP1x2.9mm, F.Cu at (140.4, 74.6)
- added U19: PTN3460, Package_DFN_QFN:QFN-56-1EP_7x7mm_P0.4mm_EP5.6x5.6mm, F.Cu at (143.2, 63.6)
- added U2: SY8120, Package_TO_SOT_SMD:TSOT-23-6, F.Cu at (85.3, 46.0)
- added U3: SY8120, Package_TO_SOT_SMD:TSOT-23-6, F.Cu at (175.2, 68.6)
- added U4: MT9700, Package_TO_SOT_SMD:SOT-23-5, F.Cu at (74.3, 43.5)
- added U6: MT9700, Package_TO_SOT_SMD:SOT-23-5, F.Cu at (64.4, 43.4)
- added U7: MT3608(SOT23-6), Package_TO_SOT_SMD:SOT-23-6, F.Cu at (101.3, 75.4)
- added U8: MT3608(SOT23-6), Package_TO_SOT_SMD:SOT-23-6, F.Cu at (101.0, 65.2)
- added U9: LGS5148, Package_TO_SOT_SMD:TSOT-23-6, F.Cu at (107.5, 65.2)
- added Y2: 12MHz, Oscillator:Oscillator_SMD_Abracon_ASE-4Pin_3.2x2.5mm, F.Cu at (98.1, 51.0)
- added Y3: 28.63636MHz, Oscillator:Oscillator_SMD_Abracon_ASE-4Pin_3.2x2.5mm, F.Cu at (139.2, 97.7)
- C68: renamed from C529; moved to F.Cu
- C71: renamed from C511; moved to B.Cu
- C86: renamed from C525; value 10uF -> 10uF/10V; footprint Capacitor_SMD:C_0603_1608Metric -> Capacitor_SMD:C_0805_2012Metric
- J2: renamed from J201; value Conn_02x05_Odd_Even -> DNP
- R11: renamed from R201; value 27 -> 27R
- R13: renamed from R306; moved to F.Cu
- R35: renamed from R509; value 0 -> 0R
- R36: renamed from R510; value 0 -> 0R
- R37: renamed from R505; value 100R 1% -> 100R/1%
- R39: renamed from R501; value 470R -> 100R/1%
- R40: renamed from R507; moved to F.Cu
- R42: renamed from R508; moved to B.Cu
- R43: renamed from R503; value 1.5K/0.5% -> 1K/1%
- R44: renamed from R504; value 1.5K/0.5% -> 1K/1%
- RN1: renamed from RN401; value 33 -> 33R / 4D02WGF330JTCE
- RN2: renamed from RN402; value 33 -> 33R / 4D02WGF330JTCE
- RN3: renamed from RN403; value 33 -> 33R / 4D02WGF330JTCE
- RN4: renamed from RN404; value 33 -> 33R / 4D02WGF330JTCE
- RN5: renamed from RN405; value 33 -> 33R / 4D02WGF330JTCE
- RN6: renamed from RN406; value 33 -> 33R / 4D02WGF330JTCE
- moved R10 58.6 mm to (83.0, 67.3)
- moved C64 51.2 mm to (185.0, 78.0)
- moved R16 50.6 mm to (187.0, 78.0), turned to 180 degrees
- moved R13 39.0 mm to (84.1, 69.7)
- moved R36 38.2 mm to (83.6, 81.1)
- moved C30 38.1 mm to (77.9, 80.4)
- moved Y1 38.1 mm to (80.6, 81.1)
- moved R11 38.1 mm to (83.7, 76.9)
- moved R35 38.1 mm to (83.7, 79.0)
- moved R12 37.6 mm to (77.9, 82.4), turned to 90 degrees
- moved J2 36.6 mm to (99.0, 90.5), turned to 90 degrees
- moved H4 26.2 mm to (152.0, 43.0)
- moved C71 20.9 mm to (122.5, 52.8), turned to -90 degrees
- moved C85 20.8 mm to (123.2, 40.5)
- moved C77 14.3 mm to (120.5, 44.5)
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- renumbered C210 to C18, C213 to C19, C215 to C20, C217 to C21, C219 to C22, C220 to C23, C211 to C24, C214 to C25, C201 to C26, C203 to C27, C204 to C28, C202 to C29, C209 to C30, C305 to C60, C306 to C61, C307 to C62, C308 to C63, C503 to C64, C501 to C65, C504 to C66, C502 to C67, C508 to C69, C510 to C70, C509 to C72, C513 to C73, C514 to C74, C512 to C75, C515 to C76, C516 to C77, C517 to C78, C518 to C79, C519 to C80, C520 to C81, C521 to C82, C522 to C83, C523 to C84, C524 to C85, C526 to C87, C527 to C88, J401 to J3, R310 to R10, R202 to R12, R309 to R14, R209 to R16, R506 to R38, R502 to R41, U502 to U12, U200 to U5, Y201 to Y1
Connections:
- net +1V1 renamed +1V0
- U5 pad A10: LVDS_EVEN_AN -> unconnected-(U5A-IO_L35N_GCLK16_0-PadA10)
- U5 pad A11: LVDS_EVEN_BN -> unconnected-(U5A-IO_L39N_0-PadA11)
- U5 pad A12: LVDS_EVEN_CN -> unconnected-(U5A-IO_L62N_VREF_0-PadA12)
- U5 pad A14: unconnected-(U200A-IO_L65N_SCP2_0-PadA14) -> VIN_HPD
- U5 pad A5: LVDS_ODD_AN -> unconnected-(U5A-IO_L2N_0-PadA5)
- U5 pad A6: LVDS_ODD_BN -> TMDS_D2P
- U5 pad A9: LVDS_ODD_CKN -> TMDS_D0P
- U5 pad B10: LVDS_EVEN_AP -> unconnected-(U5A-IO_L35P_GCLK17_0-PadB10)
- U5 pad B12: LVDS_EVEN_CP -> unconnected-(U5A-IO_L62P_0-PadB12)
- U5 pad B5: LVDS_ODD_AP -> unconnected-(U5A-IO_L2P_0-PadB5)
- U5 pad B6: LVDS_ODD_BP -> TMDS_D2N
- U5 pad C10: unconnected-(U200A-IO_L37N_GCLK12_0-PadC10) -> TMDS_CKP
- U5 pad C11: LVDS_EVEN_BP -> unconnected-(U5A-IO_L39P_0-PadC11)
- U5 pad C6: LVDS_ODD_CN -> TMDS_D1P
- U5 pad C9: LVDS_ODD_CKP -> TMDS_D0N
- U5 pad D6: LVDS_ODD_CP -> TMDS_D1N
- U5 pad E10: unconnected-(U200A-IO_L37P_GCLK13_0-PadE10) -> TMDS_CKN
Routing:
- net GND: track 227.6 -> 61.3 mm, vias 154 -> 82
- net +1V35: track 72.2 -> 16.7 mm, vias 24 -> 10
- net +DRAM_VREF: track 56.8 -> 2.64 mm, vias 5 -> 0
- net +3V3: track 103.8 -> 51.4 mm, vias 47 -> 17
- net USB_DN: track 59.3 -> 8.71 mm, vias 3 -> 1
- net USB_DP: track 58.3 -> 8.56 mm, vias 2 -> 1
- net /dp_in/VBUS: track 37.8 -> 0.00 mm, vias 5 -> 0
- net VGH: track 61.9 -> 28.4 mm, vias 2 -> 1
- net EPD_PWR_EN: track 57.1 -> 23.7 mm, vias 2 -> 1
- net /dp_in/SBU1: track 32.5 -> 0.00 mm, vias 4 -> 0
- net +5V_EPD: track 0.00 -> 31.0 mm, vias 0 -> 21
- net I2C_SCL: track 28.3 -> 0.00 mm, vias 2 -> 0
- net I2C_SDA: track 28.0 -> 0.00 mm, vias 4 -> 0
- net Net-(C609-Pad1): track 26.5 -> 0.00 mm
- net DP_PDN: track 26.4 -> 0.00 mm
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- added copper zone on In2.Cu, net +3V3
- added copper zone on F.Cu, net +5V_EPD
- added copper zone on In2.Cu, net +5V_EPD
- added copper zone on B.Cu, net GND
- added copper zone on F.Cu, net GND
- added copper zone on In1.Cu, net GND
- removed copper zone on F.Cu, net +1V0
- removed copper zone on In1.Cu, net +1V0
- removed copper zone on F.Cu, net +1V35
- removed copper zone on In1.Cu, net +1V35
- removed copper zone on In1.Cu, net +3V3
- removed copper zone on In1.Cu, net +5V
- removed copper zone on In1.Cu, net /dp_in/VBUS
- removed copper zone on In2.Cu, net GND
- removed copper zone on F.Cu, net Net-(U204-SW)
- removed copper zone on F.Cu, net Net-(U205-SW)
- removed copper zone on F.Cu, net Net-(U206-SW)
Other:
- board size 58 x 47 mm -> 60 x 60 mm
- board text added: "DDR"
- board text added: "FPGA JTAG"
- board text added: "Glider"
- board text added: "R0.8 Modos"
- board text added: "SWD"
- board text removed: "(C) 2023 Wenting/ Modos"
- board text removed: "Glider R0.6"
